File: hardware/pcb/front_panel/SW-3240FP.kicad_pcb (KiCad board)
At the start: 2 copper layers, 170.2 x 40.7 mm, 53 parts, among them J1 JTAG, J2 ESPFlash, J3 OLED, J4 FP_IO, J5 I2C, Q1 DMN2040U, SW1 PEC11R-4225F-S0024, SW2 DNP, U1 ESP32-WROOM-32D

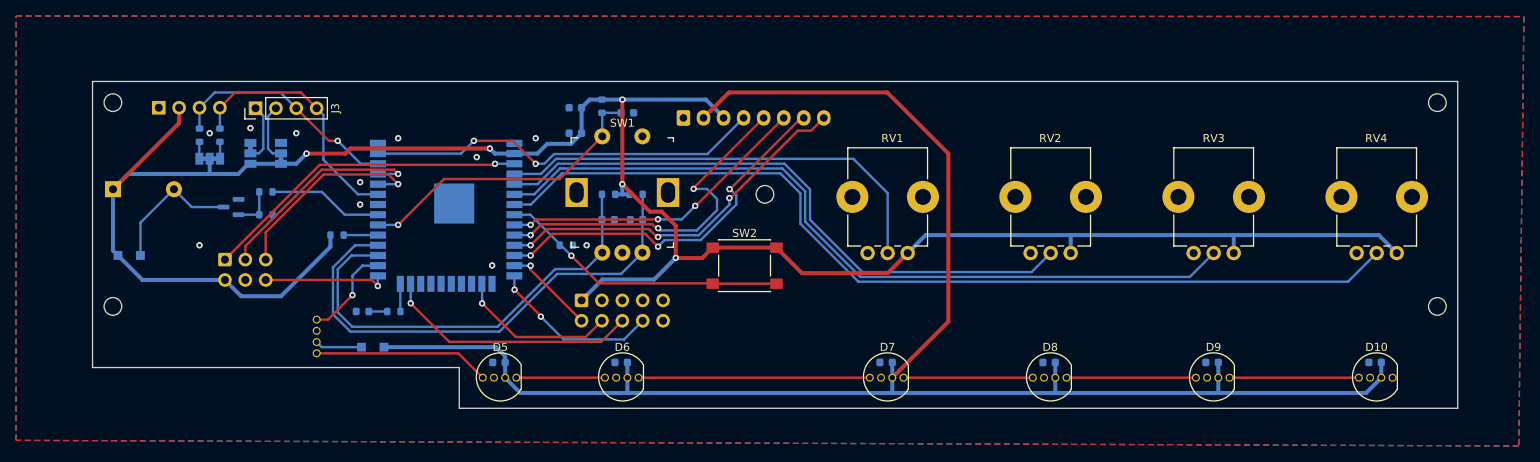
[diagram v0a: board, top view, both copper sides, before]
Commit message: redesign
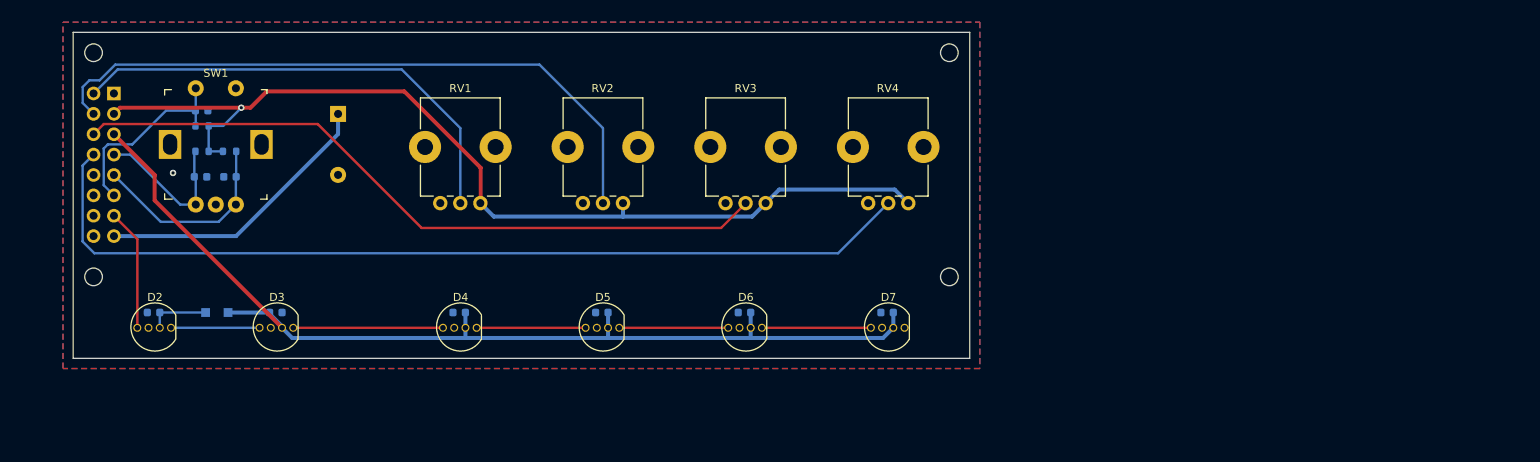
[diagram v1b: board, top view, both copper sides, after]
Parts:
- removed the C5 at (158.1, 85.1)
- removed the C6 at (142.1, 116.2)
- removed the D2 at (96.0, 102.9)
- removed the D3 at (126.4, 114.3)
- removed the D4 at (119.4, 113.0)
- removed the H1 at (175.3, 95.2)
- removed J2: ESPFlash, Connector_IDC:IDC-Header_2x03_P2.54mm_Vertical
- removed J3: OLED, SaawLib:OLED_I2C_1.3
- removed J4: FP_IO, Connector_JST:JST_XH_B8B-XH-A_1x08_P2.50mm_Vertical
- removed J5: I2C, Connector_PinHeader_2.54mm:PinHeader_1x04_P2.54mm_Vertical
- removed JP1, JP2: SolderJumper_3_Bridged12, Jumper:SolderJumper-3_P1.3mm_Bridged12_Pad1.0x1.5mm_NumberLabels
- removed JP3: SolderJumper_3_Bridged123, SaawLib:SolderJumper-3_P1.3mm_Bridged123_Pad1.0x1.5mm_NumberLabels
- removed Q1: DMN2040U, Package_TO_SOT_SMD:SOT-23
- removed R10, R4, R9: 10K, Resistor_SMD:R_0603_1608Metric
- removed R5: 10k, Resistor_SMD:R_0603_1608Metric
- removed R6, R7: 2.7K, Resistor_SMD:R_0603_1608Metric
- removed R8: 10, Resistor_SMD:R_0603_1608Metric
- removed SW2: DNP, Button_Switch_SMD:SW_Push_1P1T_NO_6x6mm_H9.5mm
- removed U1: ESP32-WROOM-32D, RF_Module:ESP32-WROOM-32
- C3: value 10uF -> 10nF
- D1: value LED -> MBR120; footprint LED_SMD:LED_0603_1608Metric -> Diode_SMD:D_SOD-123F
- H1: renamed from H2; moved to B.Cu
- H2: renamed from H3; moved to B.Cu
- H3: renamed from H4; moved to B.Cu
- H4: renamed from H5; moved to B.Cu
- J1: value JTAG -> MAIN_BOARD; footprint Connector_IDC:IDC-Header_2x05_P2.54mm_Vertical -> Connector_PinHeader_2.54mm:PinHeader_2x08_P2.54mm_Vertical
- R3: value 10k -> 10K
- moved J1 63.7 mm to (94.1, 82.7), turned to 180 degrees
- moved RV4 61.2 mm to (193.1, 96.3)
- moved C9 61.2 mm to (190.5, 110.0)
- moved D7 61.2 mm to (190.6, 111.9)
- moved H4 61.2 mm to (198.2, 77.6), turned to 180 degrees
- moved H1 60.9 mm to (198.2, 105.5), turned to 180 degrees
- moved RV3 58.7 mm to (175.3, 96.3)
- moved C8 58.6 mm to (172.7, 110.0)
- moved D6 58.6 mm to (172.8, 111.9)
- moved C4 57.1 mm to (99.0, 110.0), turned to 0 degrees
- moved RV2 56.2 mm to (157.6, 96.3)
- moved C7 56.1 mm to (154.9, 110.0)
- moved D5 56.1 mm to (155.1, 111.9)
- moved RV1 53.6 mm to (139.8, 96.3)
- moved C6 53.6 mm to (137.1, 110.0)
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- renumbered C7 to C5, C8 to C6, C9 to C7, C10 to C8, C11 to C9, D5 to D2, D6 to D3, D7 to D4, D8 to D5, D9 to D6, D10 to D7
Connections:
- BZ1 pad 1: +3V3 -> /BUZZER
- BZ1 pad 2: Net-(BZ1-Pad2) -> GND
- C3 pad 1: +3V3 -> /ENC_SW
- C4 pad 1: +3V3 -> GND
- C4 pad 2: GND -> Net-(C4-Pad2)
- D1 pad 1: GND -> Net-(C4-Pad2)
- D1 pad 2: Net-(D1-Pad2) -> +5V
- D2 pad 2: +5V -> Net-(C4-Pad2)
- D2 pad 4: Net-(D4-Pad1) (its old number) -> /LED_DATA
- J1 pad 1: +3V3 -> GND
- J1 pad 2: /MTMS -> /LVL_1
- J1 pad 3: GND -> +3V3
- J1 pad 4: /MTCK -> /LVL_2
- J1 pad 5: unconnected-(J1-Pad5) -> +5V
- J1 pad 6: /MTDO -> /LVL_3
- J1 pad 7: unconnected-(J1-Pad7) -> /ENC_A
- J1 pad 8: /MTDI -> /LVL_4
- J1 pad 9: unconnected-(J1-Pad9) -> /ENC_B
- R3 pad 1: /IO5 -> +3V3
- R3 pad 2: +3V3 -> /ENC_SW
- RV1 pad 2: /LVL_A -> /LVL_1
- RV2 pad 2: /LVL_B -> /LVL_2
- RV3 pad 2: /LVL_C -> /LVL_3
- RV4 pad 2: /LVL_D -> /LVL_4
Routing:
- net +3V3: track 280.2 -> 123.0 mm, vias 5 -> 1
- net /LVL_D: track 118.4 -> 0.00 mm
- net /LVL_4: track 0.00 -> 115.0 mm
- net /LVL_C: track 97.6 -> 0.00 mm
- net /LVL_3: track 0.00 -> 88.5 mm
- net +5V: track 212.0 -> 129.2 mm
- net /LVL_2: track 0.00 -> 82.5 mm
- net /LVL_B: track 76.7 -> 0.00 mm
- net /LVL_1: track 0.00 -> 59.3 mm
- net /LVL_A: track 56.6 -> 0.00 mm
- net /MAIN_SCL: track 49.8 -> 0.00 mm, vias 2 -> 0
- net /LINE_LEFT: track 46.9 -> 0.00 mm, vias 3 -> 0
- net /MIC: track 46.4 -> 0.00 mm, vias 3 -> 0
- net /MAIN_SDA: track 44.5 -> 0.00 mm, vias 3 -> 0
- net /EN: track 41.0 -> 0.00 mm, vias 1 -> 0
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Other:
- board size 170.2 x 40.7 mm -> 111.8 x 40.6 mm
- board text added: "SW-3240 Front Panel Rev 1"
